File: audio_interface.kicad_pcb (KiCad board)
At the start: 2 copper layers, 36 x 14 mm, 25 parts, among them IC1 ATMEGA16U2, P1 USB_A, P2 AVR-ISP, P3 OUT, P4 EAR, Q1 BC849, Q2 BC849, SW1 SW_PUSH, Y1 CSTCE16M0V53MU

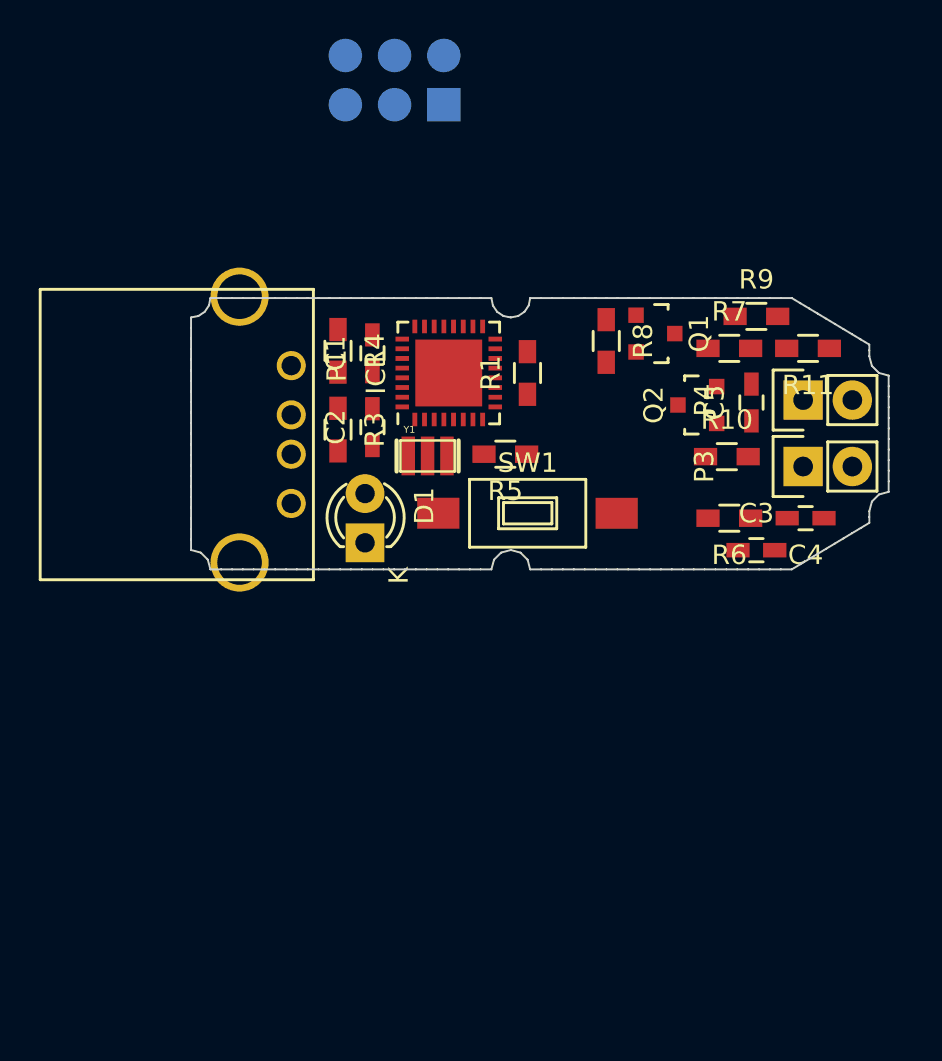
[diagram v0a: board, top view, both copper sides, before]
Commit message: update
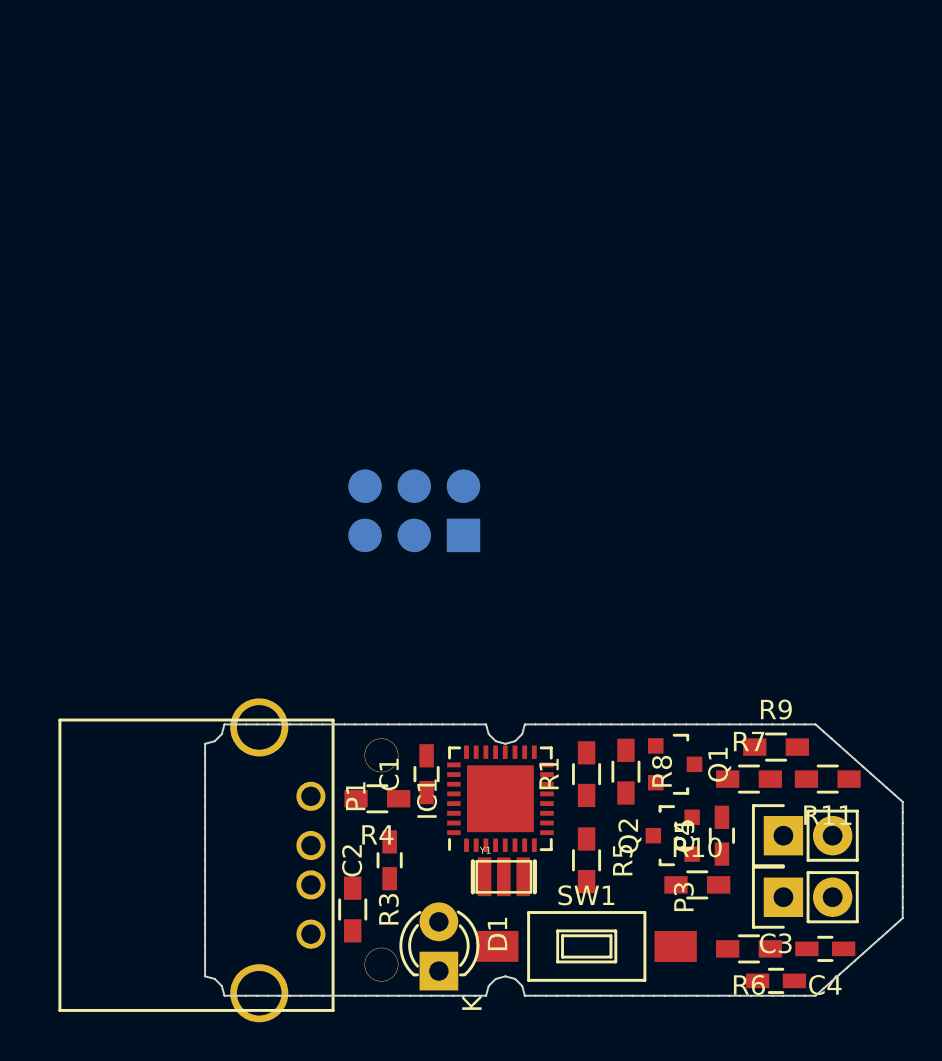
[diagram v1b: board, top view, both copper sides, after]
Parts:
- added ?: AK-S-27 Case, KaiBader:AK-S-27_Case, F.Cu at (127.0, 121.9)
- moved R3 24.8 mm to (134.6, 117.5)
- moved R4 23.2 mm to (135.9, 111.8), turned to 180 degrees
- moved SW1 22.6 mm to (146.7, 119.4)
- moved P4 22.5 mm to (156.8, 113.7)
- moved D1 22.4 mm to (139.1, 120.7)
- moved C5 22.4 mm to (153.7, 113.7)
- moved C2 22.4 mm to (136.5, 114.9)
- moved Q2 22.3 mm to (151.1, 113.7)
- moved C4 22.2 mm to (159.0, 119.5)
- moved P2 22.2 mm to (140.3, 98.2)
- moved P3 22.2 mm to (156.8, 116.8)
- moved R6 22.2 mm to (155.1, 119.5)
- moved R9 22.2 mm to (156.5, 109.1)
- moved C3 22.2 mm to (156.5, 121.2)
- moved P1 22.2 mm to (132.5, 111.6)
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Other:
- outline, holes or cut-outs redrawn
